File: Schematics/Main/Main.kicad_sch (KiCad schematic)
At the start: 3 parts, among them U1 PCM5102A, U2 PAM8403D

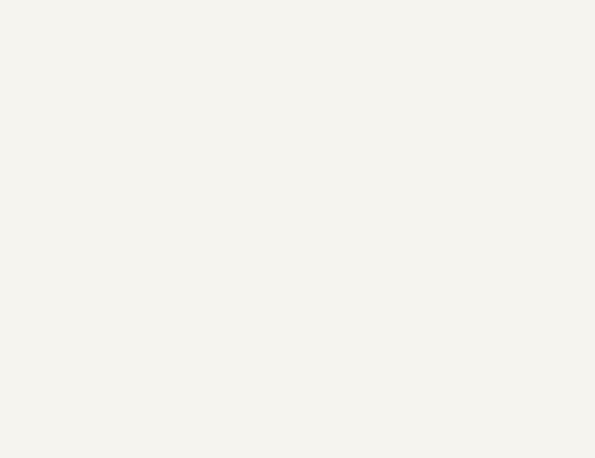
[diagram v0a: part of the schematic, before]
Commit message: Started Adding PCM5102 board schematic
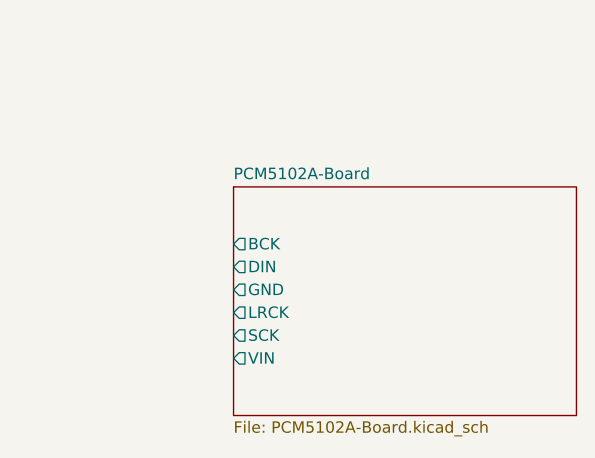
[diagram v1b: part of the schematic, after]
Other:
- added sheet PCM5102A-Board (PCM5102A-Board.kicad_sch)
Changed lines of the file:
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@@
 (kicad_sch
-	(version 20231120)
+	(version 20250114)
 	(generator "eeschema")
-	(generator_version "8.0")
+	(generator_version "9.0")
 	(paper "A4")
 	(title_block
@@
 		)
 	)
+	(sheet
+		(at 201.93 115.57)
+		(size 38.1 25.4)
+		(exclude_from_sim no)
+		(in_bom yes)
+		(on_board yes)
+		(dnp no)
+		(fields_autoplaced yes)
+		(stroke
+			(width 0.1524)
+			(type solid)
+		)
+		(fill
+			(color 0 0 0 0.0000)
+		)
+		(property "Sheetname" "PCM5102A-Board"
+			(at 201.93 114.8584 0)
+			(effects
+				(font
+					(size 1.27 1.27)
+				)
+				(justify left bottom)
+			)
+		)
+		(property "Sheetfile" "PCM5102A-Board.kicad_sch"
+			(at 201.93 141.5546 0)
+			(effects
+				(font
+					(size 1.27 1.27)
+				)
+				(justify left top)
+			)
+		)
+		(pin "BCK" output
+			(at 201.93 121.92 180)
+			(effects
+				(font
+					(size 1.27 1.27)
+				)
+				(justify left)
+			)
+		)
+		(pin "DIN" output
+			(at 201.93 124.46 180)
+			(effects
+				(font
+					(size 1.27 1.27)
+				)
+				(justify left)
+			)
+		)
+		(pin "GND" output
+			(at 201.93 127 180)
+			(effects
+				(font
+					(size 1.27 1.27)
+				)
+				(justify left)
+			)
+		)
+		(pin "LRCK" output
+			(at 201.93 129.54 180)
+			(effects
+				(font
+					(size 1.27 1.27)
+				)
+				(justify left)
+			)
+		)
+		(pin "SCK" output
+			(at 201.93 132.08 180)
+			(effects
+				(font
+					(size 1.27 1.27)
+				)
+				(justify left)
+			)
+		)
+		(pin "VIN" output
+			(at 201.93 134.62 180)
+			(effects
+				(font
+					(size 1.27 1.27)
+				)
+				(justify left)
+			)
+		)
+		(instances
+			(project "Main"
+				(path "/2b6c83b8-b6db-46e9-a845-f7ffa0649aa2"
+					(page "2")
+				)
+			)
+		)
+	)
 	(sheet_instances
 		(path "/"
@@
 		)
 	)
+	(embedded_fonts no)
 )

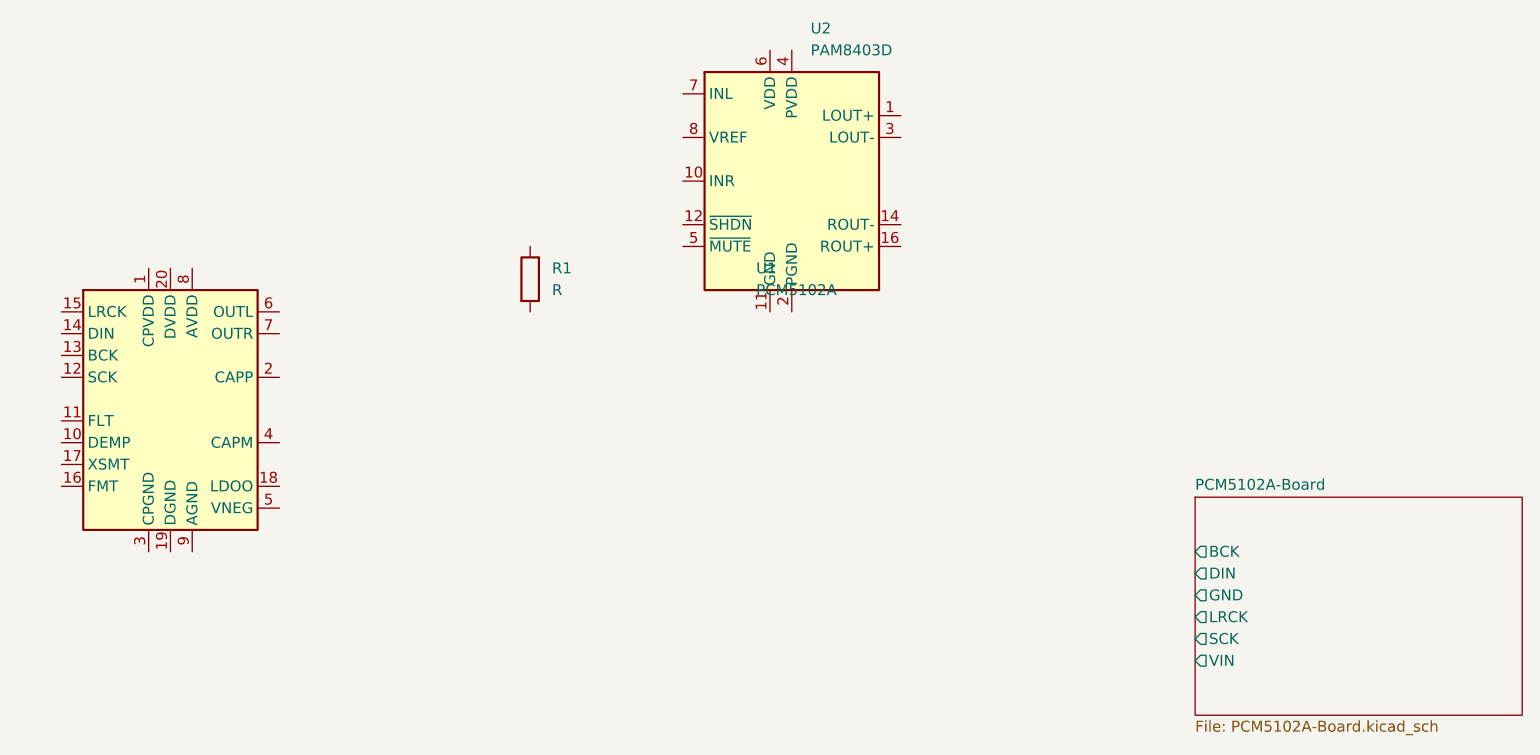
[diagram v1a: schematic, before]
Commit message: Continue on Laptop
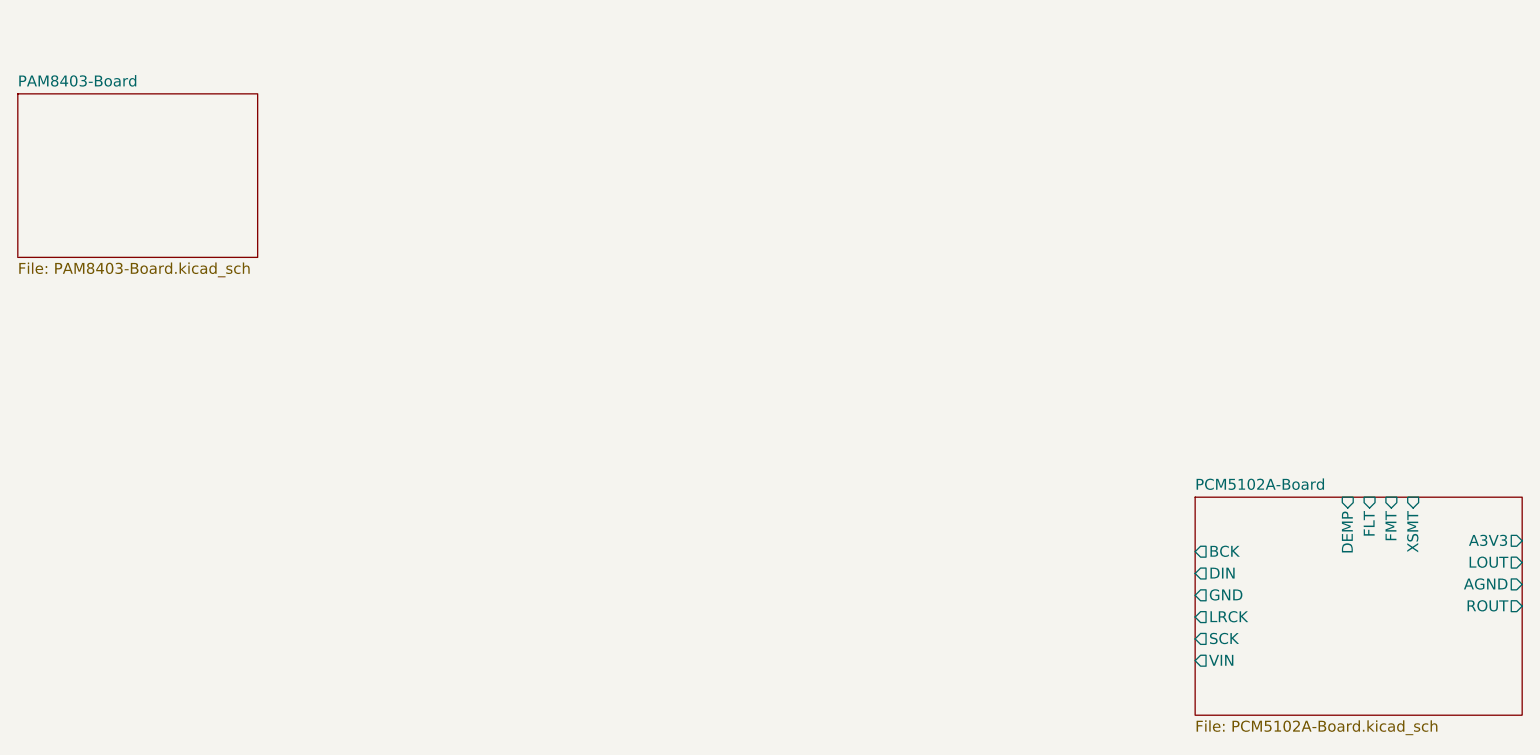
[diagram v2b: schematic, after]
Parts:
- removed R1: R, symbol Device:R
- removed U1: PCM5102A, Package_SO:TSSOP-20_4.4x6.5mm_P0.65mm, symbol Audio:PCM5102A
- removed U2: PAM8403D, Package_SO:SOP-16_3.9x9.9mm_P1.27mm, symbol Amplifier_Audio:PAM8403D
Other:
- added sheet PAM8403-Board (PAM8403-Board.kicad_sch)
- sheet PCM5102A-Board ports: added A3V3, AGND, DEMP, FLT, FMT, LOUT, ROUT, XSMT; removed none
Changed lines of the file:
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@@
 		(date "2025-02-21")
 	)
-	(symbol
-		(lib_id "Amplifier_Audio:PAM8403D")
-		(at 154.94 78.74 0)
-		(unit 1)
+	(sheet
+		(at 64.77 68.58)
+		(size 27.94 19.05)
 		(exclude_from_sim no)
 		(in_bom yes)
@@
 		(dnp no)
 		(fields_autoplaced yes)
-		(property "Reference" "U2"
-			(at 157.1341 60.96 0)
-			(effects
-				(font
-					(size 1.27 1.27)
-				)
-				(justify left)
-			)
-		)
-		(property "Value" "PAM8403D"
-			(at 157.1341 63.5 0)
-			(effects
-				(font
-					(size 1.27 1.27)
-				)
-				(justify left)
-			)
-		)
-		(property "Footprint" "Package_SO:SOP-16_3.9x9.9mm_P1.27mm"
-			(at 154.94 78.74 0)
-			(effects
-				(font
-					(size 1.27 1.27)
-				)
-				(hide yes)
-			)
-		)
-		(property "Datasheet" "https://www.diodes.com/assets/Datasheets/products_inactive_data/PAM8403.pdf"
-			(at 149.86 73.66 0)
-			(effects
-				(font
-					(size 1.27 1.27)
-				)
-				(hide yes)
-			)
-		)
-		(property "Description" "3W Filterless Class-D Stereo Audio Amplifier, SOP-16"
-			(at 154.94 78.74 0)
-			(effects
-				(font
-					(size 1.27 1.27)
-				)
-				(hide yes)
-			)
-		)
-		(pin "13"
-		)
-		(pin "11"
-		)
-		(pin "5"
-		)
-		(pin "2"
-		)
-		(pin "4"
-		)
-		(pin "16"
-		)
-		(pin "14"
-		)
-		(pin "7"
-		)
-		(pin "15"
-		)
-		(pin "6"
-		)
-		(pin "8"
-		)
-		(pin "12"
-		)
-		(pin "10"
-		)
-		(pin "3"
-		)
-		(pin "9"
-		)
-		(pin "1"
+		(stroke
+			(width 0.1524)
+			(type solid)
+		)
+		(fill
+			(color 0 0 0 0.0000)
+		)
+		(property "Sheetname" "PAM8403-Board"
+			(at 64.77 67.8684 0)
+			(effects
+				(font
+					(size 1.27 1.27)
+				)
+				(justify left bottom)
+			)
+		)
+		(property "Sheetfile" "PAM8403-Board.kicad_sch"
+			(at 64.77 88.2146 0)
+			(effects
+				(font
+					(size 1.27 1.27)
+				)
+				(justify left top)
+			)
 		)
 		(instances
-			(project ""
+			(project "Main"
 				(path "/2b6c83b8-b6db-46e9-a845-f7ffa0649aa2"
-					(reference "U2")
-					(unit 1)
-				)
-			)
-		)
-	)
-	(symbol
-		(lib_id "Audio:PCM5102A")
-		(at 82.55 104.14 0)
-		(unit 1)
-		(exclude_from_sim no)
-		(in_bom yes)
-		(on_board yes)
-		(dnp no)
-		(property "Reference" "U1"
-			(at 150.7841 88.9 0)
-			(effects
-				(font
-					(size 1.27 1.27)
-				)
-				(justify left)
-			)
-		)
-		(property "Value" "PCM5102A"
-			(at 150.7841 91.44 0)
-			(effects
-				(font
-					(size 1.27 1.27)
-				)
-				(justify left)
-			)
-		)
-		(property "Footprint" "Package_SO:TSSOP-20_4.4x6.5mm_P0.65mm"
-			(at 107.95 120.65 0)
-			(effects
-				(font
-					(size 1.27 1.27)
-				)
-				(hide yes)
-			)
-		)
-		(property "Datasheet" "https://www.ti.com/lit/ds/symlink/pcm5102a.pdf"
-			(at 82.55 104.14 0)
-			(effects
-				(font
-					(size 1.27 1.27)
-				)
-				(hide yes)
-			)
-		)
-		(property "Description" "2.1 VRMS, 112dB Audio Stereo DAC with PLL and 32-bit, 384kHz PCM Interface, TSSOP-20"
-			(at 82.55 104.14 0)
-			(effects
-				(font
-					(size 1.27 1.27)
-				)
-				(hide yes)
-			)
-		)
-		(pin "2"
-		)
-		(pin "18"
-		)
-		(pin "12"
-		)
-		(pin "20"
-		)
-		(pin "8"
-		)
-		(pin "5"
-		)
-		(pin "7"
-		)
-		(pin "4"
-		)
-		(pin "1"
-		)
-		(pin "13"
-		)
-		(pin "9"
-		)
-		(pin "3"
-		)
-		(pin "15"
-		)
-		(pin "6"
-		)
-		(pin "10"
-		)
-		(pin "14"
-		)
-		(pin "19"
-		)
-		(pin "11"
-		)
-		(pin "16"
-		)
-		(pin "17"
-		)
-		(instances
-			(project ""
-				(path "/2b6c83b8-b6db-46e9-a845-f7ffa0649aa2"
-					(reference "U1")
-					(unit 1)
-				)
-			)
-		)
-	)
-	(symbol
-		(lib_id "Device:R")
-		(at 124.46 90.17 0)
-		(unit 1)
-		(exclude_from_sim no)
-		(in_bom yes)
-		(on_board yes)
-		(dnp no)
-		(fields_autoplaced yes)
-		(property "Reference" "R1"
-			(at 127 88.8999 0)
-			(effects
-				(font
-					(size 1.27 1.27)
-				)
-				(justify left)
-			)
-		)
-		(property "Value" "R"
-			(at 127 91.4399 0)
-			(effects
-				(font
-					(size 1.27 1.27)
-				)
-				(justify left)
-			)
-		)
-		(property "Footprint" ""
-			(at 122.682 90.17 90)
-			(effects
-				(font
-					(size 1.27 1.27)
-				)
-				(hide yes)
-			)
-		)
-		(property "Datasheet" "~"
-			(at 124.46 90.17 0)
-			(effects
-				(font
-					(size 1.27 1.27)
-				)
-				(hide yes)
-			)
-		)
-		(property "Description" "Resistor"
-			(at 124.46 90.17 0)
-			(effects
-				(font
-					(size 1.27 1.27)
-				)
-				(hide yes)
-			)
-		)
-		(pin "2"
-		)
-		(pin "1"
-		)
-		(instances
-			(project ""
-				(path "/2b6c83b8-b6db-46e9-a845-f7ffa0649aa2"
-					(reference "R1")
-					(unit 1)
+					(page "3")
 				)
 			)
@@
 			)
 		)
+		(pin "A3V3" output
+			(at 240.03 120.65 0)
+			(effects
+				(font
+					(size 1.27 1.27)
+				)
+				(justify right)
+			)
+		)
+		(pin "AGND" output
+			(at 240.03 125.73 0)
+			(effects
+				(font
+					(size 1.27 1.27)
+				)
+				(justify right)
+			)
+		)
+		(pin "DEMP" input
+			(at 219.71 115.57 90)
+			(effects
+				(font
+					(size 1.27 1.27)
+				)
+				(justify right)
+			)
+		)
+		(pin "FLT" input
+			(at 222.25 115.57 90)
+			(effects
+				(font
+					(size 1.27 1.27)
+				)
+				(justify right)
+			)
+		)
+		(pin "FMT" input
+			(at 224.79 115.57 90)
+			(effects
+				(font
+					(size 1.27 1.27)
+				)
+				(justify right)
+			)
+		)
+		(pin "LOUT" output
+			(at 240.03 123.19 0)
+			(effects
+				(font
+					(size 1.27 1.27)
+				)
+				(justify right)
+			)
+		)
+		(pin "ROUT" output
+			(at 240.03 128.27 0)
+			(effects
+				(font
+					(size 1.27 1.27)
+				)
+				(justify right)
+			)
+		)
+		(pin "XSMT" input
+			(at 227.33 115.57 90)
+			(effects
+				(font
+					(size 1.27 1.27)
+				)
+				(justify right)
+			)
+		)
